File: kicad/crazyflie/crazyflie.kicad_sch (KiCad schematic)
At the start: 7 parts, among them J1 Conn_01x10_Female, J2 Conn_01x10_Female, J8 Conn_01x04_Socket, M1 Conn_01x03_Socket, M2 Conn_01x03_Socket, M3 Conn_01x03_Socket, M4 Conn_01x03_Socket

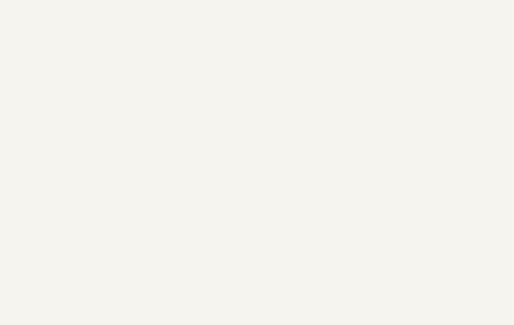
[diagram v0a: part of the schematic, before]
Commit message: modified:   kicad/crazyflie/crazyflie.kicad_pcb
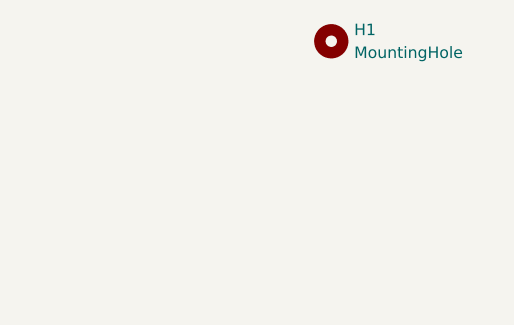
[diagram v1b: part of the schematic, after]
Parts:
- added H1: MountingHole, MountingHole:MountingHole_5.3mm_M5_ISO7380_Pad_TopOnly, symbol Mechanical:MountingHole
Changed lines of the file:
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@@
+	)
+	(symbol
+		(lib_id "Mechanical:MountingHole")
+		(at 166.37 58.42 0)
+		(unit 1)
+		(exclude_from_sim no)
+		(in_bom no)
+		(on_board yes)
+		(dnp no)
+		(fields_autoplaced yes)
+		(property "Reference" "H1"
+			(at 168.91 57.1499 0)
+			(effects
+				(font
+					(size 1.27 1.27)
+				)
+				(justify left)
+			)
+		)
+		(property "Value" "MountingHole"
+			(at 168.91 59.6899 0)
+			(effects
+				(font
+					(size 1.27 1.27)
+				)
+				(justify left)
+			)
+		)
+		(property "Footprint" "MountingHole:MountingHole_5.3mm_M5_ISO7380_Pad_TopOnly"
+			(at 166.37 58.42 0)
+			(effects
+				(font
+					(size 1.27 1.27)
+				)
+				(hide yes)
+			)
+		)
+		(property "Datasheet" "~"
+			(at 166.37 58.42 0)
+			(effects
+				(font
+					(size 1.27 1.27)
+				)
+				(hide yes)
+			)
+		)
+		(property "Description" "Mounting Hole without connection"
+			(at 166.37 58.42 0)
+			(effects
+				(font
+					(size 1.27 1.27)
+				)
+				(hide yes)
+			)
+		)
+		(instances
+			(project ""
+				(path "/afb8e687-4a13-41a1-b8c0-89a749e897fe"
+					(reference "H1")
+					(unit 1)
+				)
+			)
+		)
 	)
 	(symbol

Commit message: modified:   kicad/crazyflie/crazyflie.kicad_pcb
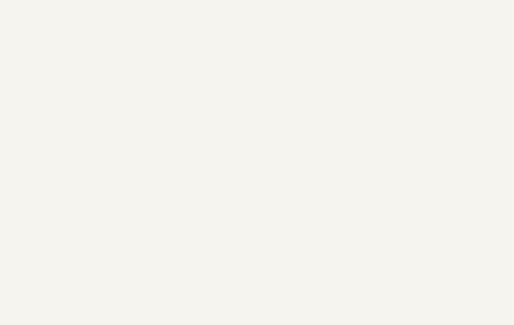
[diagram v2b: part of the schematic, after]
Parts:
- removed H1: MountingHole, MountingHole:MountingHole_5.3mm_M5_ISO7380_Pad_TopOnly, symbol Mechanical:MountingHole
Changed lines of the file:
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@@
-	)
-	(symbol
-		(lib_id "Mechanical:MountingHole")
-		(at 166.37 58.42 0)
-		(unit 1)
-		(exclude_from_sim no)
-		(in_bom no)
-		(on_board yes)
-		(dnp no)
-		(fields_autoplaced yes)
-		(property "Reference" "H1"
-			(at 168.91 57.1499 0)
-			(effects
-				(font
-					(size 1.27 1.27)
-				)
-				(justify left)
-			)
-		)
-		(property "Value" "MountingHole"
-			(at 168.91 59.6899 0)
-			(effects
-				(font
-					(size 1.27 1.27)
-				)
-				(justify left)
-			)
-		)
-		(property "Footprint" "MountingHole:MountingHole_5.3mm_M5_ISO7380_Pad_TopOnly"
-			(at 166.37 58.42 0)
-			(effects
-				(font
-					(size 1.27 1.27)
-				)
-				(hide yes)
-			)
-		)
-		(property "Datasheet" "~"
-			(at 166.37 58.42 0)
-			(effects
-				(font
-					(size 1.27 1.27)
-				)
-				(hide yes)
-			)
-		)
-		(property "Description" "Mounting Hole without connection"
-			(at 166.37 58.42 0)
-			(effects
-				(font
-					(size 1.27 1.27)
-				)
-				(hide yes)
-			)
-		)
-		(instances
-			(project ""
-				(path "/afb8e687-4a13-41a1-b8c0-89a749e897fe"
-					(reference "H1")
-					(unit 1)
-				)
-			)
-		)
 	)
 	(symbol
